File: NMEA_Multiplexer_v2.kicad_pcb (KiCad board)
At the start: 2 copper layers, 45 x 65 mm, 94 parts, among them J1 USB, J2 Port 1, J3 Port 2, J4 Port 3, J5 Port 4, J6 Port 5, J7 12V, J8 DEBUG UART, SW1 Reset, U1 ATSAMG55J19A-AU, U2 XR32330, U3 XR32330, U4 LF33ABDT-TR, U5 HM-11, Y1 32.768k

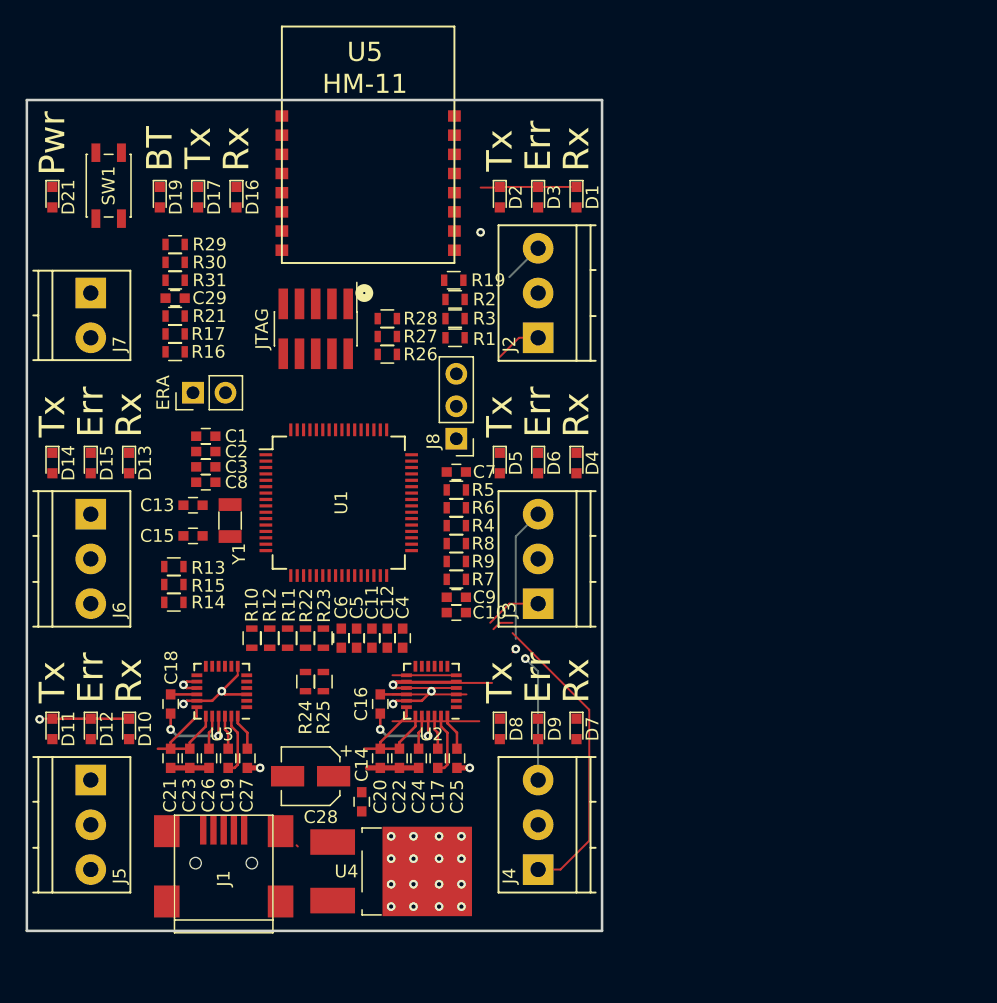
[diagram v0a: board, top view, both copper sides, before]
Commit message: Bottom half completed
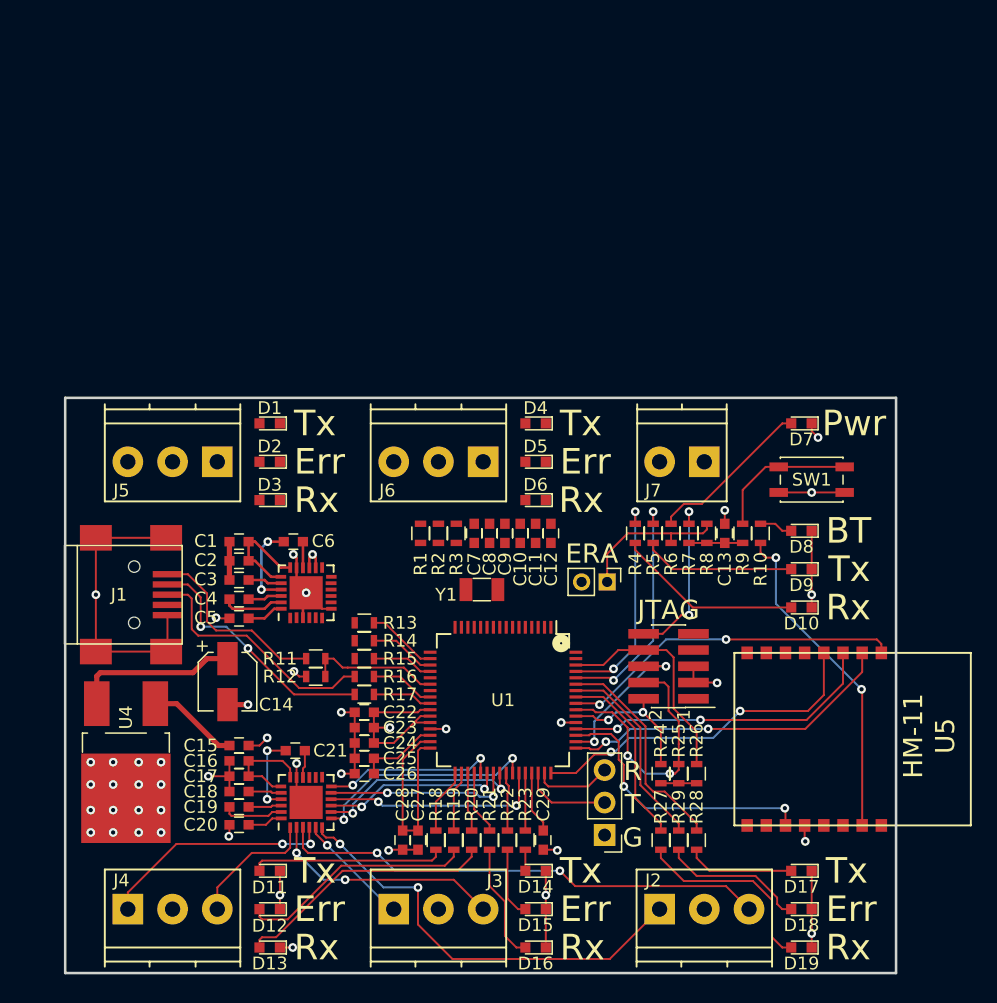
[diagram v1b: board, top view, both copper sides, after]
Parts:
- removed ERA: ERASE, Pin_Headers:Pin_Header_Straight_1x02_Pitch2.54mm
- added JP1: ERASE, Pin_Headers:Pin_Header_Straight_1x02_Pitch2.00mm, F.Cu at (245.4, 121.6)
- D1: renamed from D11; value Tx 3 (green) -> Tx 3 (gReen)
- D11: renamed from D8; value Tx (green) -> Tx (gReen)
- D12: renamed from D9; value Err 2 (red) -> ERr 2 (reD)
- D14: renamed from D5; value Tx 1 (green) -> Tx 1 (gReen)
- D15: renamed from D6; value Err 1 (red) -> ERr 1 (reD)
- D17: renamed from D2; value Tx 0 (green) -> Tx 0 (gReen)
- D18: renamed from D3; value Err 0 (red) -> ERr 0 (reD)
- D2: renamed from D12; value Err 3 (red) -> ERr 3 (reD)
- D4: renamed from D14; value Tx 4 (green) -> Tx 4 (gReen)
- D5: renamed from D15; value Err 4 (red) -> ERr 4 (reD)
- D8: renamed from D19; value BT Con (blue) -> BT Cxon (blue)
- D9: renamed from D17; value Tx BT (green) -> Tx BT (gReen)
- J2: value Port 1 -> PoRt 1
- J3: value Port 2 -> PoRt 2
- J4: value Port 3 -> PoRt 3
- J5: value Port 4 -> PoRt 4
- J6: value Port 5 -> PoRt 5
- U2: renamed from U3; footprint Housings_DFN_QFN:QFN-24_4x4mm_Pitch0.5mm_NoMask -> MaxNil:QFN-24_4x4mm_Pitch0.5mm_NoMask
- U3: renamed from U2; footprint Housings_DFN_QFN:QFN-24_4x4mm_Pitch0.5mm_NoMask -> MaxNil:QFN-24_4x4mm_Pitch0.5mm_NoMask
- moved D19 61.3 mm to (260.6, 150.2), turned to 180 degrees
- moved D7 61.2 mm to (260.6, 109.2), turned to 180 degrees
- moved SW1 59.6 mm to (261.4, 113.6), turned to 180 degrees
- moved D18 59.4 mm to (260.6, 147.2), turned to 180 degrees
- moved U5 59.3 mm to (264.1, 133.9), turned to 270 degrees
- moved D17 57.7 mm to (260.6, 144.2), turned to 180 degrees
- moved D8 56.6 mm to (260.6, 117.6), turned to 180 degrees
- moved D9 55.4 mm to (260.6, 120.6), turned to 180 degrees
- moved D10 54.6 mm to (260.6, 123.6), turned to 180 degrees
- moved R9 49.8 mm to (256.0, 117.8), turned to 90 degrees
- moved J7 49.8 mm to (253.0, 112.2), turned to 180 degrees
- moved C13 46.8 mm to (254.6, 117.8), turned to 90 degrees
- moved R8 46.7 mm to (253.2, 117.8), turned to 270 degrees
- moved R29 45.8 mm to (251.0, 141.8), turned to 270 degrees
- moved J2 45.7 mm to (249.5, 147.2), turned to 0 degrees
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- renumbered C21 to C1, C3 to C10, C2 to C11, C1 to C12, C29 to C13, C28 to C14, C14 to C15, C20 to C16, C22 to C17, C24 to C18, C17 to C19, C23 to C2, C25 to C20, C16 to C21, C6 to C22, C11 to C23, C12 to C24, C9 to C25, C10 to C26, C4 to C27, C5 to C28, C7 to C29, C26 to C3, C19 to C4, C27 to C5, C18 to C6, C15 to C7, C13 to C8, C8 to C9, D16 to D10, D7 to D13, D4 to D16, D1 to D19, D10 to D3, D13 to D6, D21 to D7, JTAG to J9, R15 to R1, R19 to R10, R24 to R11, R25 to R12, R10 to R13, R11 to R14, R12 to R15, R22 to R16, R23 to R17, R9 to R18, R8 to R19, R14 to R2, R7 to R20, R6 to R21, R5 to R22, R4 to R23, R28 to R24, R27 to R25, R3 to R27, R1 to R28, R2 to R29, R13 to R3, R16 to R4, R17 to R5, R21 to R6, R31 to R7, R30 to R8, R29 to R9
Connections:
- net /CTS0 renamed /CxTS0
- net /LED_BT_CON renamed /LED_BT_CxON
- net /TCK renamed /TCxK
- D1 pad 2: Net-(D11-Pad2) -> Net-(D1-Pad2)
- D11 pad 2: Net-(D8-Pad2) (its old number) -> Net-(D11-Pad2)
- D12 pad 2: Net-(D9-Pad2) (its old number) -> Net-(D12-Pad2)
- D14 pad 2: Net-(D5-Pad2) -> Net-(D14-Pad2)
- D15 pad 2: Net-(D6-Pad2) (its old number) -> Net-(D15-Pad2)
- D16 pad 2: Net-(D4-Pad2) -> Net-(D16-Pad2)
- D17 pad 2: Net-(D2-Pad2) -> Net-(D17-Pad2)
- D18 pad 2: Net-(D3-Pad2) -> Net-(D18-Pad2)
- D19 pad 2: Net-(D1-Pad2) -> Net-(D19-Pad2)
- D2 pad 2: Net-(D12-Pad2) -> Net-(D2-Pad2)
- D3 pad 2: Net-(D10-Pad2) (its old number) -> Net-(D3-Pad2)
- D4 pad 2: Net-(D14-Pad2) -> Net-(D4-Pad2)
- D5 pad 2: Net-(D15-Pad2) -> Net-(D5-Pad2)
- R1 pad 1: /LED_4_ERR -> /LED_4_TX
- R1 pad 2: Net-(D15-Pad2) -> Net-(D4-Pad2)
- R13 pad 1: /LED_3_RX -> /LED_3_TX
- R13 pad 2: Net-(D10-Pad2) (its old number) -> Net-(D1-Pad2)
- R14 pad 1: /LED_3_TX -> /LED_3_ERR
- R14 pad 2: Net-(D11-Pad2) -> Net-(D2-Pad2)
- R15 pad 1: /LED_3_ERR -> /LED_3_RX
- R15 pad 2: Net-(D12-Pad2) -> Net-(D3-Pad2)
- R18 pad 1: /LED_2_ERR -> /LED_2_TX
- R18 pad 2: Net-(D9-Pad2) (its old number) -> Net-(D11-Pad2)
- R19 pad 1: /LED_2_TX -> /LED_2_ERR
- R19 pad 2: Net-(D8-Pad2) (its old number) -> Net-(D12-Pad2)
- R2 pad 1: /LED_4_TX -> /LED_4_ERR
- R2 pad 2: Net-(D14-Pad2) -> Net-(D5-Pad2)
- R21 pad 1: /LED_1_ERR -> /LED_1_RX
- R21 pad 2: Net-(D6-Pad2) (its old number) -> Net-(D16-Pad2)
- R22 pad 1: /LED_1_TX -> /LED_1_ERR
- R22 pad 2: Net-(D5-Pad2) -> Net-(D15-Pad2)
- R23 pad 1: /LED_1_RX -> /LED_1_TX
- R23 pad 2: Net-(D4-Pad2) -> Net-(D14-Pad2)
- R24 pad 2: /TDI -> /TMS
- R26 pad 2: /TMS -> /TDI
- R27 pad 1: /LED_0_ERR -> /LED_0_RX
- R27 pad 2: Net-(D3-Pad2) -> Net-(D19-Pad2)
- R28 pad 1: /LED_0_RX -> /LED_0_TX
- R28 pad 2: Net-(D1-Pad2) -> Net-(D17-Pad2)
- R29 pad 1: /LED_0_TX -> /LED_0_ERR
- R29 pad 2: Net-(D2-Pad2) -> Net-(D18-Pad2)
- U1 pad 18: /LED_3_RX -> /LED_3_TX
- U1 pad 20: Net-(U1-Pad20) -> /LED_3_RX
- U1 pad 21: /LED_3_TX -> Net-(U1-Pad21)
- U1 pad 33: /LED_2_RX -> /LED_2_TX
- U1 pad 35: /LED_2_TX -> /LED_2_RX
- U1 pad 60: /LED_BT_RX -> /LED_BT_TX
- U1 pad 61: /LED_BT_TX -> /LED_BT_RX
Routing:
- net GND: track 65.0 -> 124.8 mm, vias 23 -> 42
- net +3V3: track 32.0 -> 78.7 mm
- net /RX2: track 3.18 -> 38.5 mm, vias 0 -> 2
- net /TX2: track 3.62 -> 34.2 mm, vias 0 -> 2
- net /TXD0: track 0.00 -> 27.2 mm, vias 0 -> 2
- net /CxTS0: track 0.00 -> 26.9 mm, vias 0 -> 2
- net /RXD0: track 0.00 -> 26.4 mm, vias 0 -> 2
- net /LED_BT_CxON: track 0.00 -> 25.9 mm, vias 0 -> 2
- net /RTS0: track 0.00 -> 24.8 mm, vias 0 -> 2
- net /BT_RESET_N: track 0.00 -> 22.0 mm, vias 0 -> 2
- net /TCxK: track 0.00 -> 20.5 mm, vias 0 -> 2
- net Net-(D13-Pad2): track 0.00 -> 20.4 mm
- net Net-(J1-Pad2): track 0.00 -> 19.6 mm, vias 0 -> 2
- net Net-(J1-Pad3): track 0.00 -> 19.5 mm
- net (no net): track 19.4 -> 0.00 mm, vias 2 -> 0
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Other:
- board size 45 x 65 mm -> 65 x 45 mm
- board text added: "1"
- board text added: "2"
- board text added: "ERA"
- board text added: "G"
- board text added: "JTAG"
- board text added: "R"
- board text added: "T"
